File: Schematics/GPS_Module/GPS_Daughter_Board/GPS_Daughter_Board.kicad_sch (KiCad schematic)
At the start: 17 parts, among them J4 25SH-B-06-TR, U3 SAM-M10Q, U8 LM66100DCKR

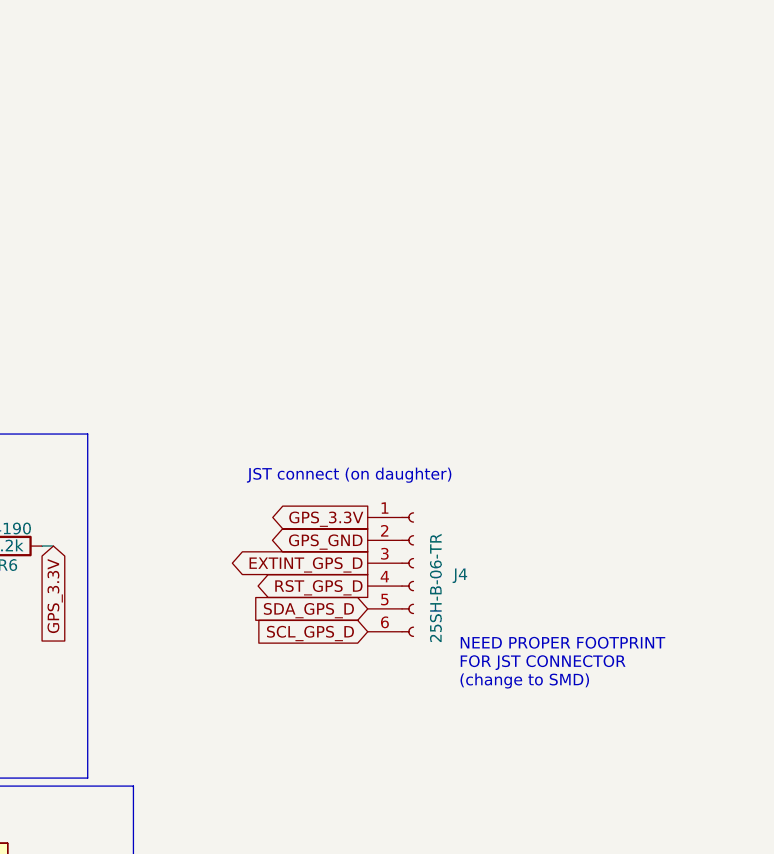
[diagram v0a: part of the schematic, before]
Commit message: starting daughter board PCB layout
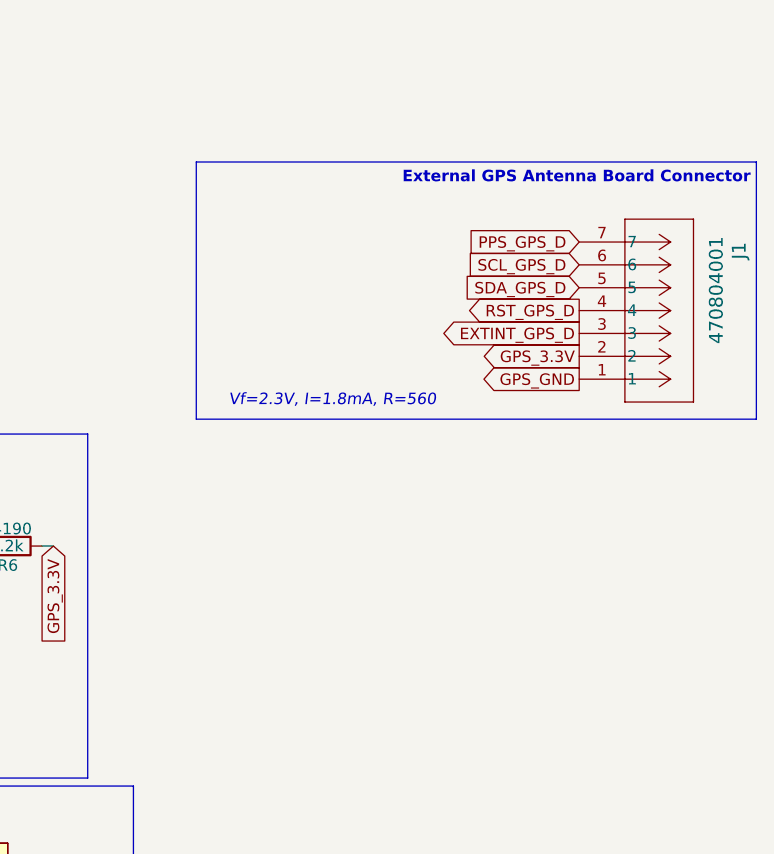
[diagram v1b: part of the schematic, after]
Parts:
- removed J4: 25SH-B-06-TR, Connector_PinHeader_2.54mm:PinHeader_1x06_P2.54mm_Horizontal, symbol Connector:Conn_01x06_Socket
- added J1: 470804001, footprints:CONN_47080-4001_MOL_SATA, symbol CONN_47080-4001_MOL_SATA:470804001
- C22: footprint Capacitor_THT:CP_Radial_D12.5mm_P7.50mm -> CB5R5334HF-ZJP:CB5R5334HF-ZJP
- U8: footprint LMR66100:SC-70-6 -> LMR66100:SC-70-6_Handsoldering
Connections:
- net EXTINT_GPS_D: now also J1.3
- net GPS_3.3V: now also J1.2
- net GPS_GND: now also J1.1
- net PPS_GPS_D: now also J1.7
- net RST_GPS_D: now also J1.4
- net SCL_GPS_D: now also J1.6
- net SDA_GPS_D: now also J1.5
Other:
- note added: "External GPS Antenna Board Connector"
- note added: "Vf=2.3V, I=1.8mA, R=560"
- note removed: "JST connect (on daughter)"
- note removed: "NEED PROPER FOOTPRINT FOR JST CONNECTOR (change to SMD)"
